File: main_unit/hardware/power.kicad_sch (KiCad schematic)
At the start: 17 parts, among them U2 LD39200PU33R

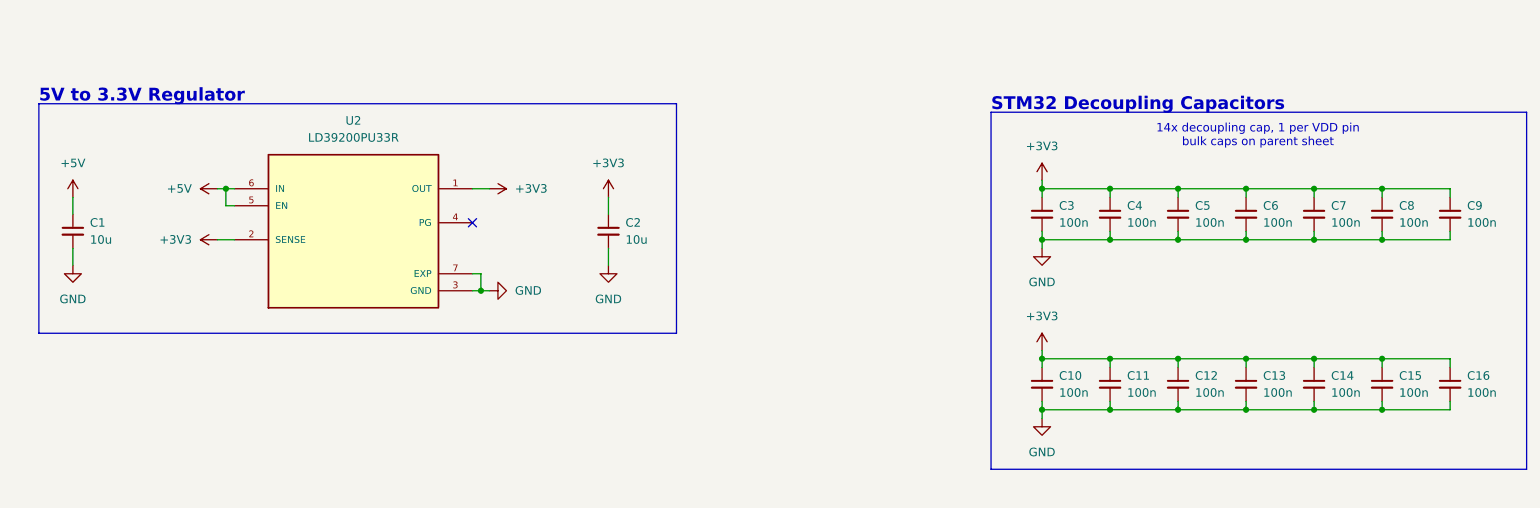
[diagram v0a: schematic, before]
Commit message: main_unit/hardware: Add in input power filtering and ST-Link connector
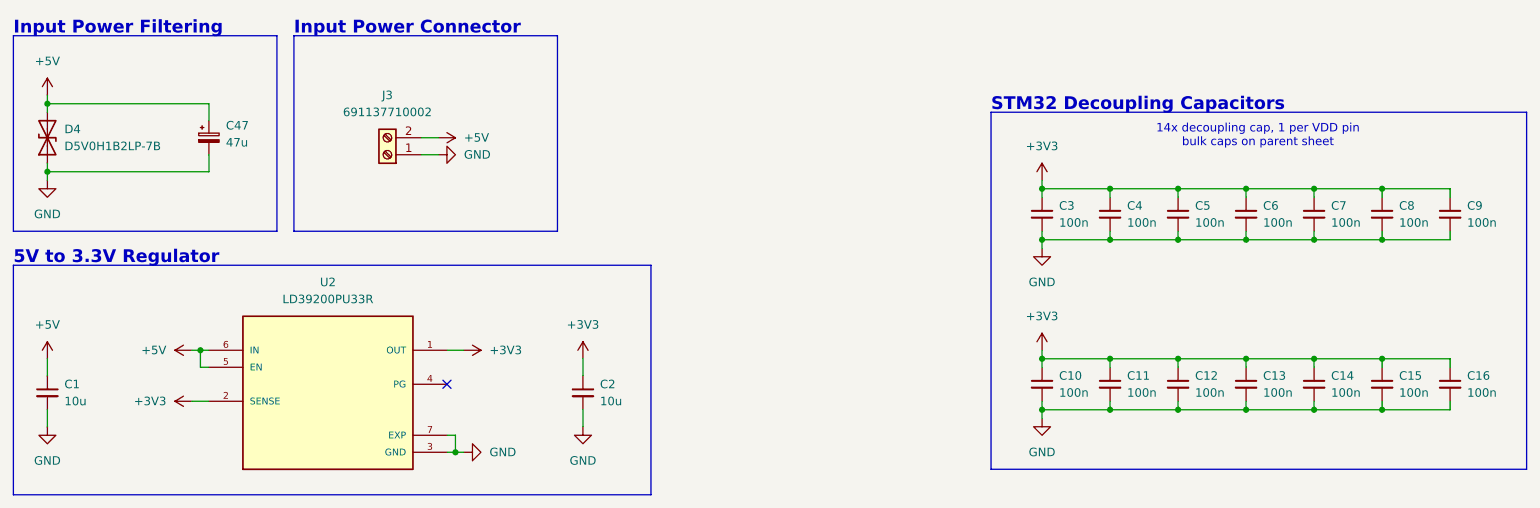
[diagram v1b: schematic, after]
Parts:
- added C47: 47u, 865080342006:WCAP-ASLI_5X5.5_DXL_, symbol Device:C_Polarized_Small
- added D4: D5V0H1B2LP-7B, Diode_SMD:D_0402_1005Metric, symbol Device:D_TVS
- added J3: 691137710002, 691137710002:691137710002, symbol Connector:Screw_Terminal_01x02
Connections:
- net +5V: now also C47.1, D4.2 (A2), J3.2 (Pin_2)
- net GND: now also C47.2, D4.1 (A1), J3.1 (Pin_1)
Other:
- note added: "Input Power Connector"
- note added: "Input Power Filtering"
- moved on the sheet: C1, C2, U2
